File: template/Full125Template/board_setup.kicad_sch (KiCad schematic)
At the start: 17 parts, among them J102 Input, J103 Output, J104 Power

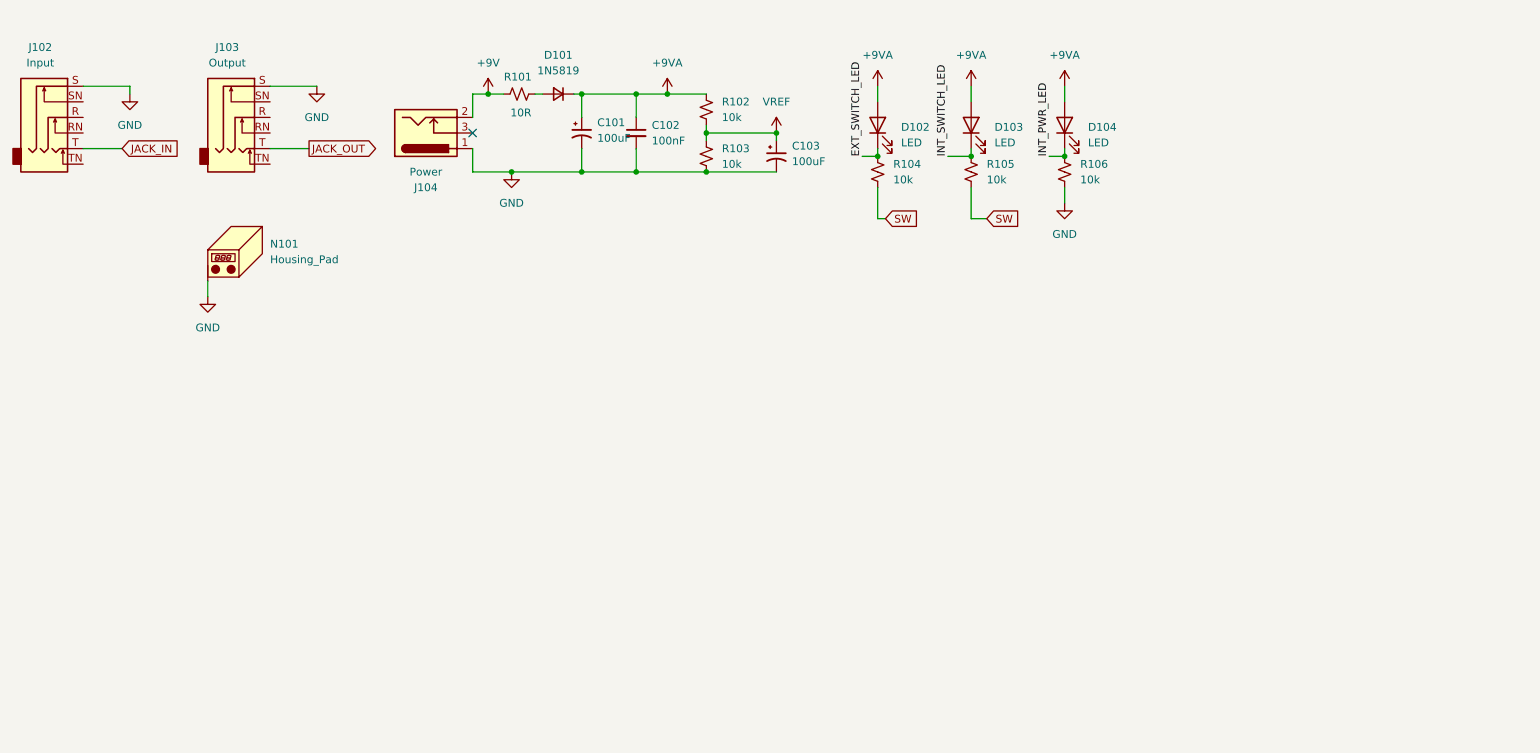
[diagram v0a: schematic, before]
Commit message: Update Full 125B template
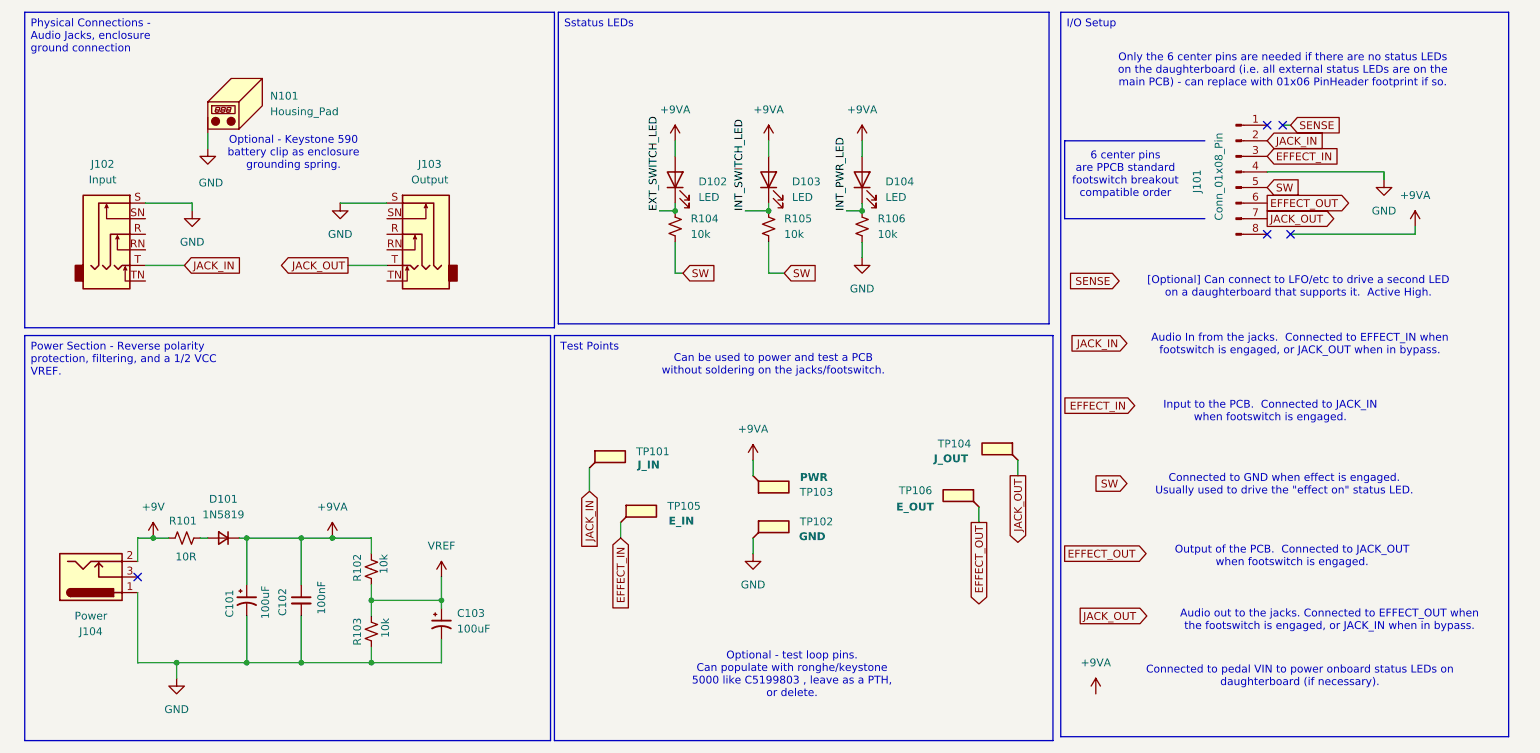
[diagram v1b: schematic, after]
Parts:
- added J101: Conn_01x08_Pin, Connector_PinSocket_2.54mm:PinSocket_1x08_P2.54mm_Vertical, symbol Connector:Conn_01x08_Pin
- added TP101, TP102, TP103, TP104, TP105, TP106: TestPoint_Flag, TestPoint:TestPoint_Keystone_5000-5004_Miniature, symbol Connector:TestPoint_Flag
- D102, J102, J103, J104: now left out of the parts list
- D103: LCSC (none) -> C84256
- D104: LCSC (none) -> C2297
- N101: LCSC (none) -> C3029553
- R101: LCSC (none) -> C22859
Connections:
- net +9VA: now also TP103.1
- net GND: now also J101.4 (Pin_4), TP102.1
- net JACK_IN: now also J101.2 (Pin_2), TP101.1
- net JACK_OUT: now also J101.7 (Pin_7), TP104.1
- net SW: now also J101.5 (Pin_5)
- new net EFFECT_IN: J101.3 (Pin_3), TP105.1
- new net EFFECT_OUT: J101.6 (Pin_6), TP106.1
- no-connect marks 1 -> 5
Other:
- note added: "6 center pins are PPCB standard footswitch breakout compatible order"
- note added: "Audio In from the jacks. Connected to EFFECT_IN when footswitch is engaged, or JACK_OUT when in bypass."
- note added: "Audio out to the jacks. Connected to EFFECT_OUT when the footswitch is engaged, or JACK_IN when in bypass."
- note added: "Can be used to power and test a PCB without soldering on the jacks/footswitch."
- note added: "Connected to GND when effect is engaged. Usually used to drive the "effect on" status LED."
- note added: "Connected to pedal VIN to power onboard status LEDs on daughterboard (if necessary)."
- note added: "Input to the PCB. Connected to JACK_IN when footswitch is engaged."
- note added: "Only the 6 center pins are needed if there are no status LEDs on the daughterboard (i.e. all external status LEDs are on the main PCB) - can replace with 01x06 PinHeader footprint if so."
- note added: "Optional - Keystone 590 battery clip as enclosure grounding spring."
- note added: "Optional - test loop pins. Can populate with ronghe/keystone 5000 like C5199803 , leave as a PTH, or delete."
- note added: "Output of the PCB. Connected to JACK_OUT when footswitch is engaged."
- note added: "[Optional] Can connect to LFO/etc to drive a second LED on a daughterboard that supports it. Active High."
- moved on the sheet: C101, C102, C103, D101, D102, D103, D104, J102, J103, J104, N101, R101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
